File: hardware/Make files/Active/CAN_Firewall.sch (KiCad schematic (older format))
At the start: 65 parts, among them CON1 BARREL_JACK, CON2 AVR-JTAG-10, CON3 AVR-AW-6, J1 +5V_SRC, J2 DB9, J3 DB9, P1 USB_OTG, P2 USB_OTG, P3 DIAG Port, SW1 SPST, SW2 SPST, SW3 SPST, U1 AT32UC3C, U2 FT232RL-SSOP, U3 MC78M05CDT, U4 SMF05, U5 MCP25625, U6 MCP25625, X1 TXC

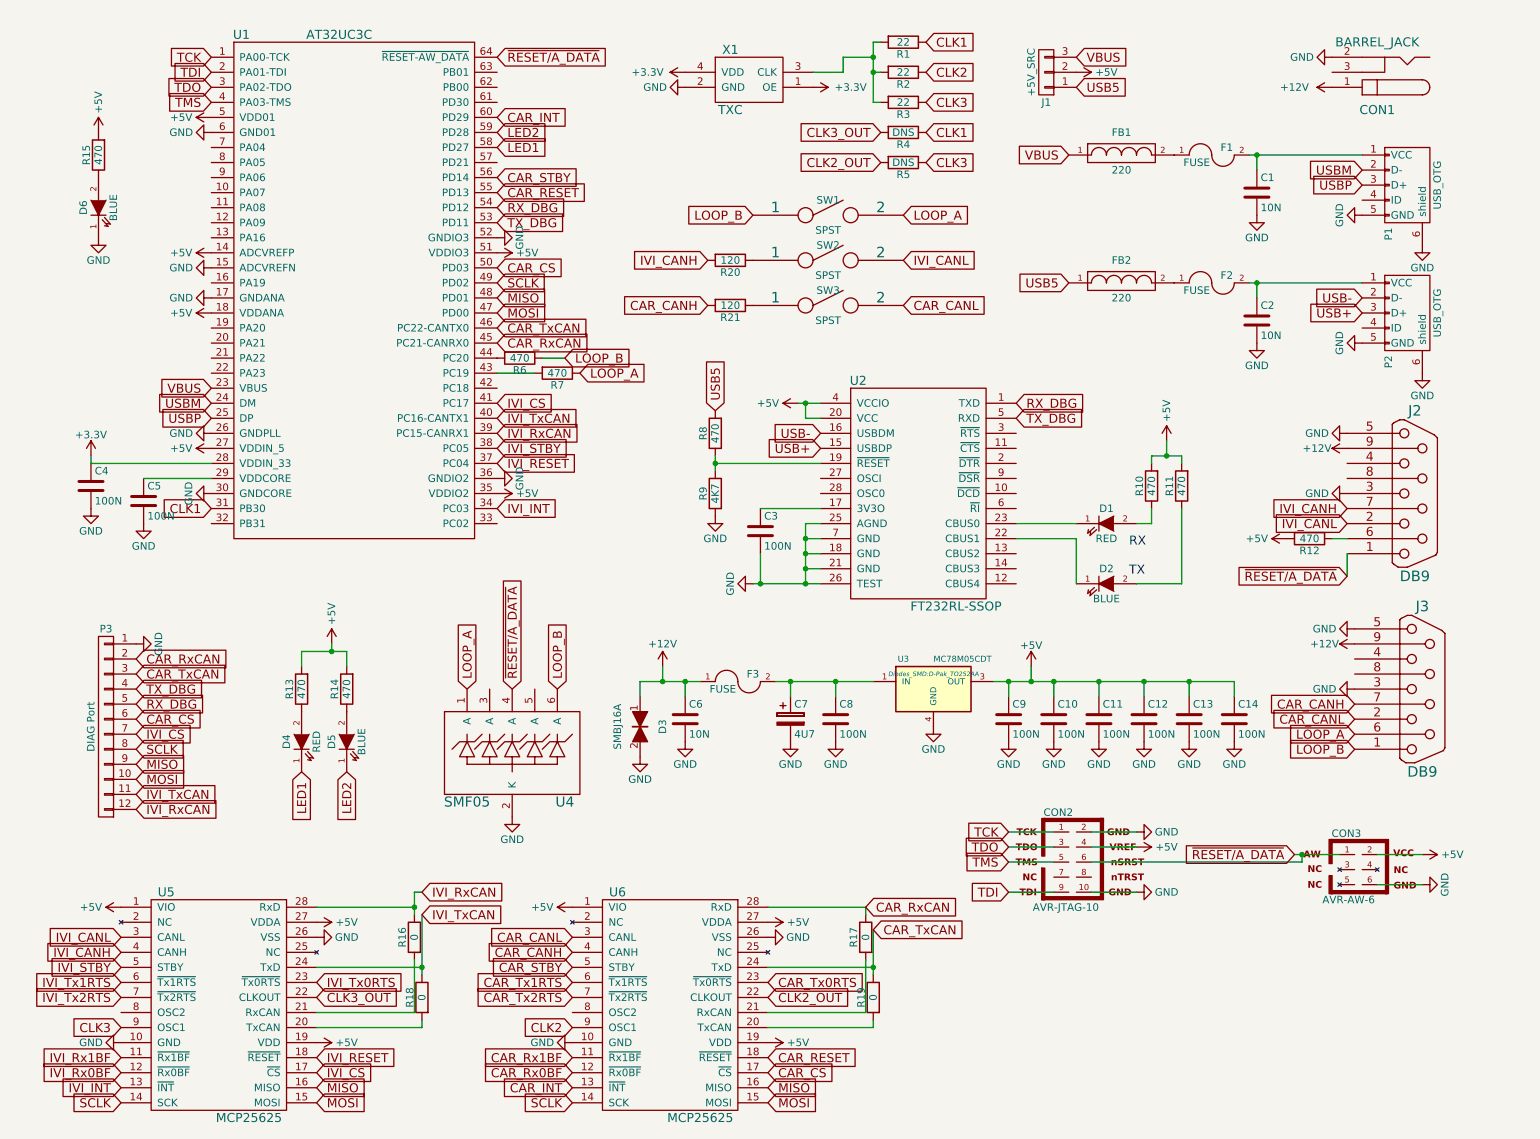
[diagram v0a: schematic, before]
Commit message: progress towards V1.2
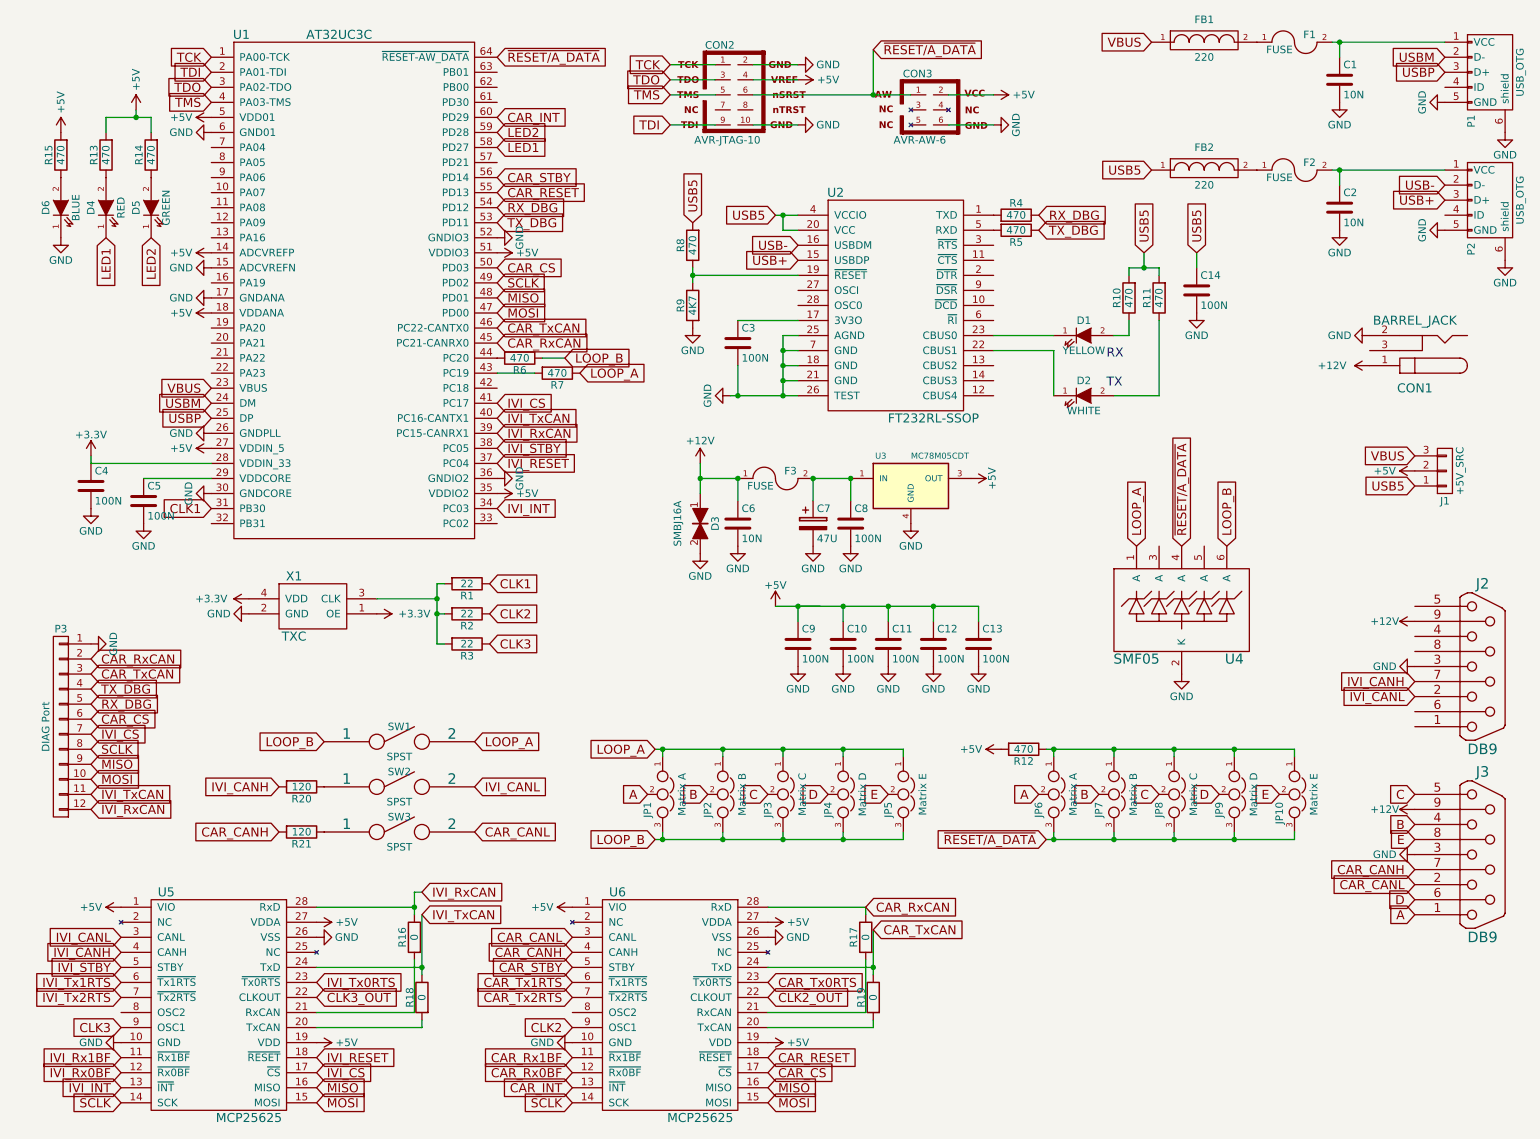
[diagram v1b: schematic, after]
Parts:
- added JP1, JP6: Matrix A, Connect:GS3, symbol JUMPER3
- added JP10, JP5: Matrix E, Connect:GS3, symbol JUMPER3
- added JP2, JP7: Matrix B, Connect:GS3, symbol JUMPER3
- added JP3, JP8: Matrix C, Connect:GS3, symbol JUMPER3
- added JP4, JP9: Matrix D, Connect:GS3, symbol JUMPER3
- C1, C2, C6: Mouser (none) -> 77-VJ0603Y103KXACBC
- C10, C11, C12, C13, C14, C3, C4, C5, C8, C9: Mouser (none) -> 581-06035C104KAT2A
- C7: value 4U7 -> 47U; footprint Capacitors_Tantalum_SMD:TantalC_SizeA_EIA-3216_Reflow -> Capacitors_SMD:c_elec_6.3x5.3; Mouser (none) -> 140-VE470M1ETR0605
- CON1: Mouser (none) -> 502-RAPC722X
- CON3: Mouser (none) -> 855-M20-9980346
- D1: value RED -> YELLOW; Mouser (none) -> 630-HSMY-C170
- D2: value BLUE -> WHITE; Mouser (none) -> 859-LTW-170ZDC
- D3: Mouser (none) -> 511-SMBJ16A
- D4: Mouser (none) -> 630-HSMH-C170
- D5: value BLUE -> GREEN; Mouser (none) -> 630-HSMG-C170
- D6: Mouser (none) -> 630-HSMR-C170
- F1, F2, F3: Mouser (none) -> 530-0ZCH0050FF2G
- FB1, FB2: Mouser (none) -> 810-MPZ1608S221ATA00
- J1: Mouser (none) -> 855-M20-9990346
- J2, J3: Mouser (none) -> 523-L77-DE09S
- P1, P2: Mouser (none) -> 656-DX4R005JJ2R1800
- P3: Mouser (none) -> 855-M20-9991246
- R1, R2, R3: Mouser (none) -> 71-CRCW0603-22.1-E3
- R10, R11, R12, R13, R14, R15, R6, R7, R8: Mouser (none) -> 71-CRCW0603-470-E3
- R16, R17, R18, R19: Mouser (none) -> 71-CRCW0603-0-E3
- R20, R21: Mouser (none) -> 71-CRCW0603-120-E3
- R4, R5: value DNS -> 470; Mouser (none) -> 71-CRCW0603-470-E3
- R9: Mouser (none) -> 71-CRCW0603-4.7K-E3
- SW1, SW2, SW3: Mouser (none) -> 653-A6TN-1104
- U1: Mouser (none) -> 556-AT32UC3C2512CA2T
- U2: Mouser (none) -> 895-FT232RL
- U3: Mouser (none) -> 511-L78M05CDT-TR
- U4: Mouser (none) -> 863-SMF05CT2G
- U5, U6: Mouser (none) -> MCP25625-E/SS
- X1: Mouser (none) -> 634-501BAA16M0000CAG
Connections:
- net +5V: no longer C14.1, R10.2, R11.2, U2.20 (VCC), U2.4 (VCCIO)
- net CLK1: no longer R4.1
- net CLK2_OUT: no longer R5.2
- net CLK3: no longer R5.1
- net CLK3_OUT: no longer R4.2
- net GND: no longer J2.5, J3.5
- net LOOP_A: now also JP1.1, JP2.1, JP3.1, JP4.1, JP5.1; no longer J3.6 (P6)
- net LOOP_B: now also JP1.3, JP2.3, JP3.3, JP4.3, JP5.3; no longer J3.1
- net RX_DBG: now also R4.1; no longer U2.1 (TXD)
- net TX_DBG: now also R5.1; no longer U2.5 (RXD)
- net USB5: now also C14.1, R10.2, R11.2, U2.20 (VCC), U2.4 (VCCIO)
- net ~RESET/A_DATA: now also JP10.3, JP6.3, JP7.3, JP8.3, JP9.3; no longer J2.1
- net at J2.6 (P6): no longer R12.1
- net B: now reaches J3.4
- net B: now also JP2.2, JP7.2
- net E: now reaches J3.8 (P8)
- net E: now also JP10.2, JP5.2
- new net: JP10.1, JP6.1, JP7.1, JP8.1, JP9.1, R12.1
- new net: R4.2, U2.1 (TXD)
- new net: R5.2, U2.5 (RXD)
- new net A: J3.1, JP1.2, JP6.2
- new net C: J3.5, JP3.2, JP8.2
- new net D: J3.6 (P6), JP4.2, JP9.2
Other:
- moved on the sheet: C1, C10, C11, C12, C13, C14, C2, C3, C6, C7, C8, C9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
